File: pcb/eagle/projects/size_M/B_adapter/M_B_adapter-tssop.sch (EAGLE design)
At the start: 16 parts

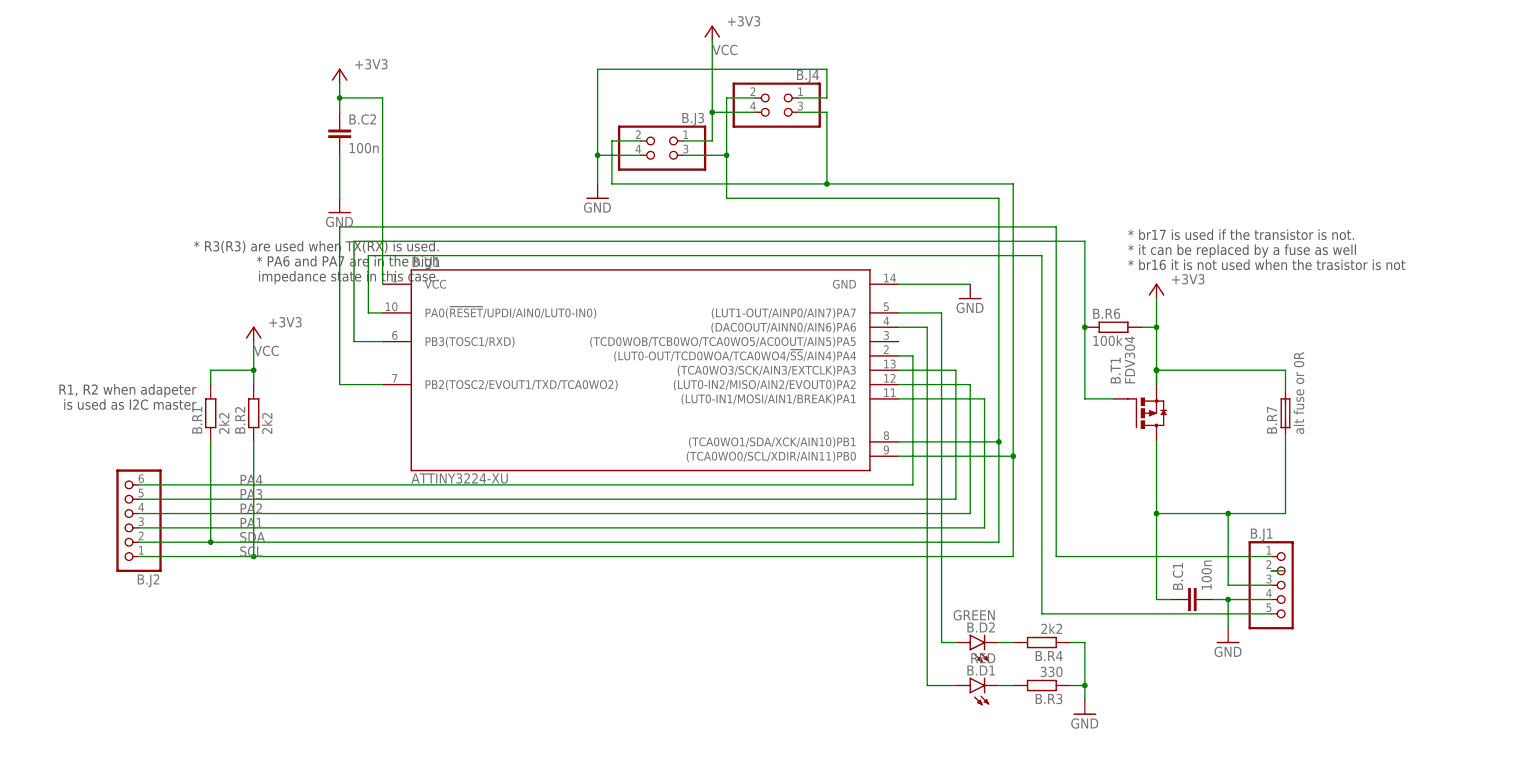
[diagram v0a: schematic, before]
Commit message: PCB v9
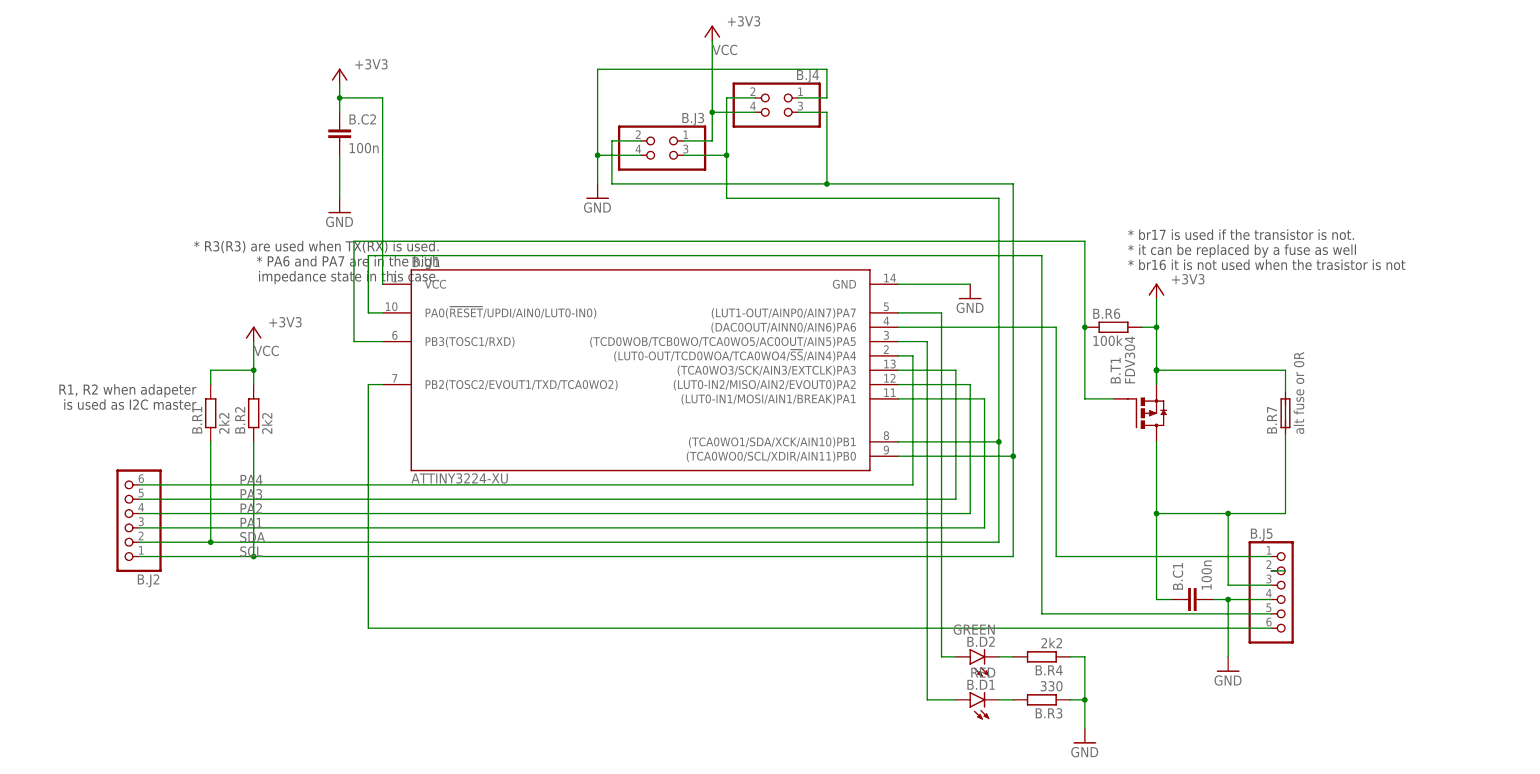
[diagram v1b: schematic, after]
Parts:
- removed B.J1: (no value), pinhead2:PINHD-1X5
- added B.J5: (no value), pinhead2:PINHD-1X6
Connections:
- new net PA6: B.J5.1, B.U1.(DAC0OUT/AINN0/AIN6)PA6
- net GND: now also B.J5.4; no longer B.J1.4
- net N$3: now also B.J5.3; no longer B.J1.3
- net N$5: now also B.U1.(TCD0WOB/TCB0WO/TCA0WO5/AC0OUT/AIN5)PA5; no longer B.U1.(DAC0OUT/AINN0/AIN6)PA6
- net PB2: now also B.J5.6; no longer B.J1.1
- net UPDI: now also B.J5.5; no longer B.J1.5
- net VBAT: now also B.J5.2; no longer B.J1.2
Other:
- moved on the sheet: B.D1, B.D2, B.R3, B.R4
